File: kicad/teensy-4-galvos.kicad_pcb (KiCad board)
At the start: 2 copper layers, 72 x 40 mm, 25 parts, among them J1 +15 G -15, J2 AudioJack3_SwitchTR, J5 x out, J6 y out, J7 405nm, U1 TL072, U2 X galvo, U3 Y TL072, U4 Teensy4.0

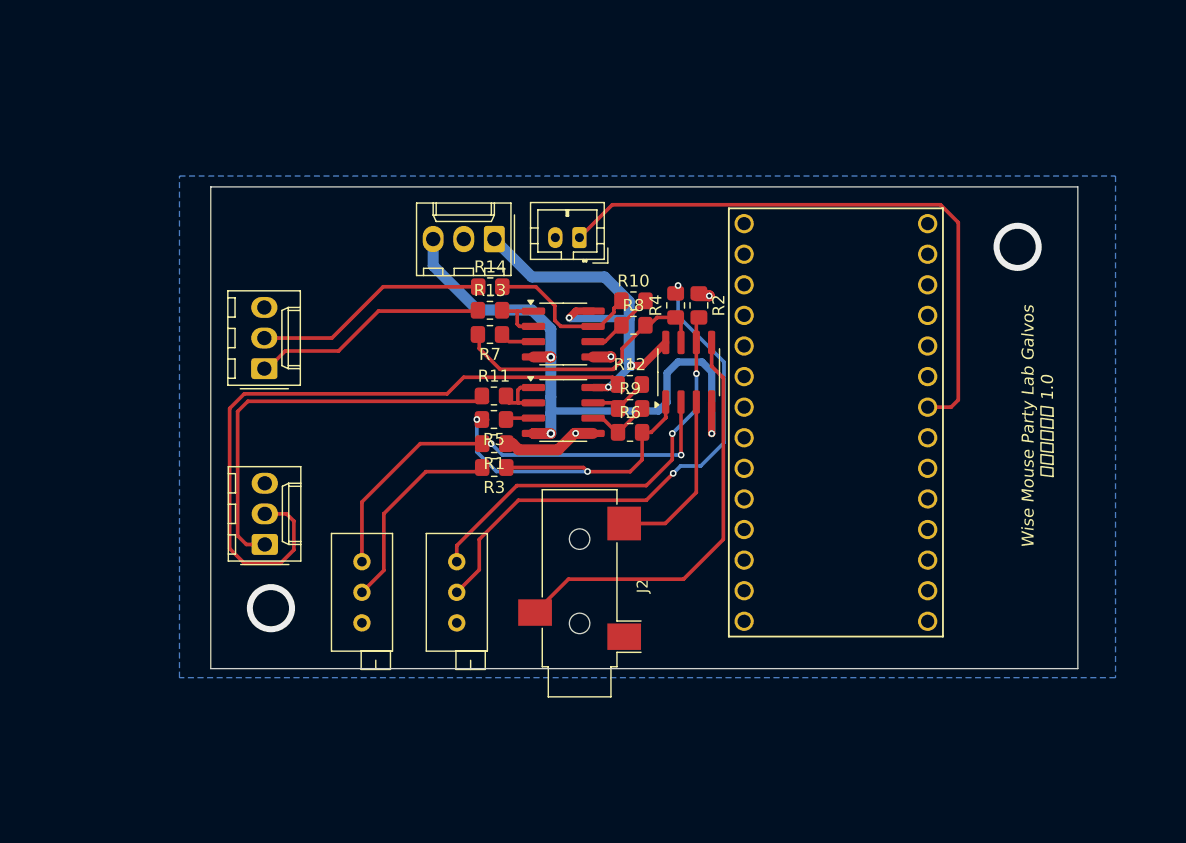
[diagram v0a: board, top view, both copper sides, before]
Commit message: Update KiCad board files
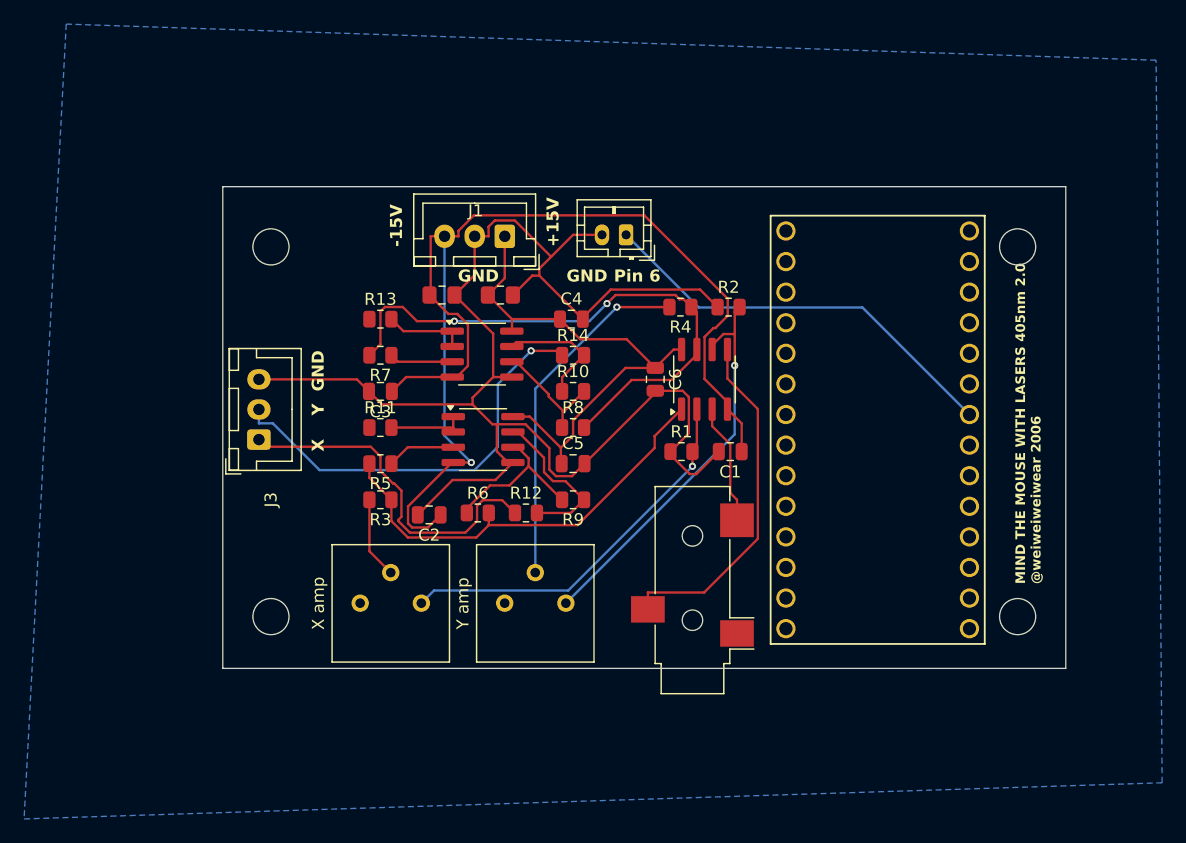
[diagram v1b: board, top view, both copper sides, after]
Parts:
- removed J5: x out, Connector_Molex:Molex_KK-254_AE-6410-03A_1x03_P2.54mm_Vertical
- removed J6: y out, Connector_Molex:Molex_KK-254_AE-6410-03A_1x03_P2.54mm_Vertical
- added C1: 0.1uF, Capacitor_SMD:C_0805_2012Metric, F.Cu at (103.1, 62.0)
- added C2: 0.1uF, Capacitor_SMD:C_0805_2012Metric, F.Cu at (78.1, 67.3)
- added C3: 0.1uF, Capacitor_SMD:C_0805_2012Metric, F.Cu at (74.1, 57.0)
- added C4: 0.1uF, Capacitor_SMD:C_0805_2012Metric, F.Cu at (90.0, 51.0)
- added C5: 0.1uF, Capacitor_SMD:C_0805_2012Metric, F.Cu at (90.1, 63.0)
- added C6: 0.1uF, Capacitor_SMD:C_0805_2012Metric, F.Cu at (96.9, 56.0)
- added C7: 10uF, Capacitor_SMD:C_0805_2012Metric_Pad1.18x1.45mm_HandSolder, F.Cu at (79.2, 49.0)
- added C8: 10uF, Capacitor_SMD:C_0805_2012Metric_Pad1.18x1.45mm_HandSolder, F.Cu at (84.0, 49.0)
- added J3: +15 G -15, Connector_JST:JST_XH_B3B-XH-A_1x03_P2.50mm_Vertical, F.Cu at (64.0, 61.0)
- J1: footprint Connector_Molex:Molex_KK-254_AE-6410-03A_1x03_P2.54mm_Vertical -> Connector_JST:JST_XH_B3B-XH-A_1x03_P2.50mm_Vertical
- R1, R10, R11, R12, R13, R14, R2, R3, R4, R5, R6, R7, R8, R9: footprint Resistor_SMD:R_0805_2012Metric_Pad1.20x1.40mm_HandSolder -> Resistor_SMD:R_0805_2012Metric
- X amp: renamed from RV1; footprint Potentiometer_THT:Potentiometer_Bourns_3296X_Horizontal -> Potentiometer_THT:Potentiometer_Bourns_3386P_Vertical
- Y amp: renamed from RV2; footprint Potentiometer_THT:Potentiometer_Bourns_3296X_Horizontal -> Potentiometer_THT:Potentiometer_Bourns_3386P_Vertical
- moved R1 15.6 mm to (99.1, 62.0), turned to 0 degrees
- moved R6 14.3 mm to (82.2, 67.1)
- moved R12 13.7 mm to (86.2, 67.1)
- moved R5 10.1 mm to (74.1, 63.0)
- moved R8 9.86 mm to (90.1, 60.0)
- moved R3 9.83 mm to (74.1, 66.0)
- moved R11 9.79 mm to (74.1, 60.0)
- moved Y amp 9.69 mm to (89.5, 74.6)
- moved J2 9.38 mm to (100.0, 73.5)
- moved R7 9.26 mm to (74.1, 54.0)
- moved R13 9.13 mm to (74.1, 51.0)
- moved R10 9.04 mm to (90.1, 57.0)
- moved R9 8.94 mm to (90.1, 66.0), turned to 180 degrees
- moved R14 8.93 mm to (90.1, 54.0)
- moved U2 7.08 mm to (82.6, 61.0)
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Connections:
- R11 pad 1: Net-(J5-Pin_1) -> unconnected-(R11-Pad1)
- R13 pad 1: Net-(J6-Pin_1) -> unconnected-(R13-Pad1)
- U4 pad 1: GND -> unconnected-(U4-GND-Pad1)
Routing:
- net GND: track 10.6 -> 122.5 mm, vias 3 -> 0
- net -15V: track 50.4 -> 94.3 mm, vias 3 -> 1
- net Net-(J5-Pin_1): track 34.0 -> 0.00 mm
- net Net-(J3-Pin_1): track 56.7 -> 29.3 mm
- net Net-(R4-Pad1): track 22.9 -> 47.8 mm, vias 0 -> 2
- net Net-(J6-Pin_1): track 19.7 -> 0.00 mm
- net /laser en: track 50.7 -> 34.7 mm
- net Net-(J3-Pin_2): track 19.5 -> 35.2 mm, vias 0 -> 1
- net Net-(R4-Pad2): track 44.3 -> 29.2 mm, vias 2 -> 1
- net Net-(R3-Pad2): track 17.0 -> 6.78 mm
- net +15V: track 33.8 -> 43.4 mm, vias 3 -> 0
- net Net-(R12-Pad2): track 4.68 -> 13.3 mm
- net Net-(U2B--): track 5.38 -> 13.2 mm
- net Net-(U1A--): track 38.3 -> 32.1 mm, vias 2 -> 1
- net Ax_Ring_OUT: track 34.9 -> 29.1 mm
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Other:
- board size 72 x 40 mm -> 70 x 40 mm
- board text added: "+15V"
- board text added: "-15V"
- board text added: "GND"
- board text added: "MIND THE MOUSE WITH LASERS 405nm 2.0 @weiweiweiwear 2006"
- board text added: "Pin 6"
- board text added: "X"
- board text added: "Y"
- board text removed: "Wise Mouse Party Lab Galvos 雷射振鏡系統 1.0"
